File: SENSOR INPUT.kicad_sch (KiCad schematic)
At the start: 18 parts, among them J1 Screw_Terminal_01x02, J4 Screw_Terminal_01x03, U3 MAX31855KASA

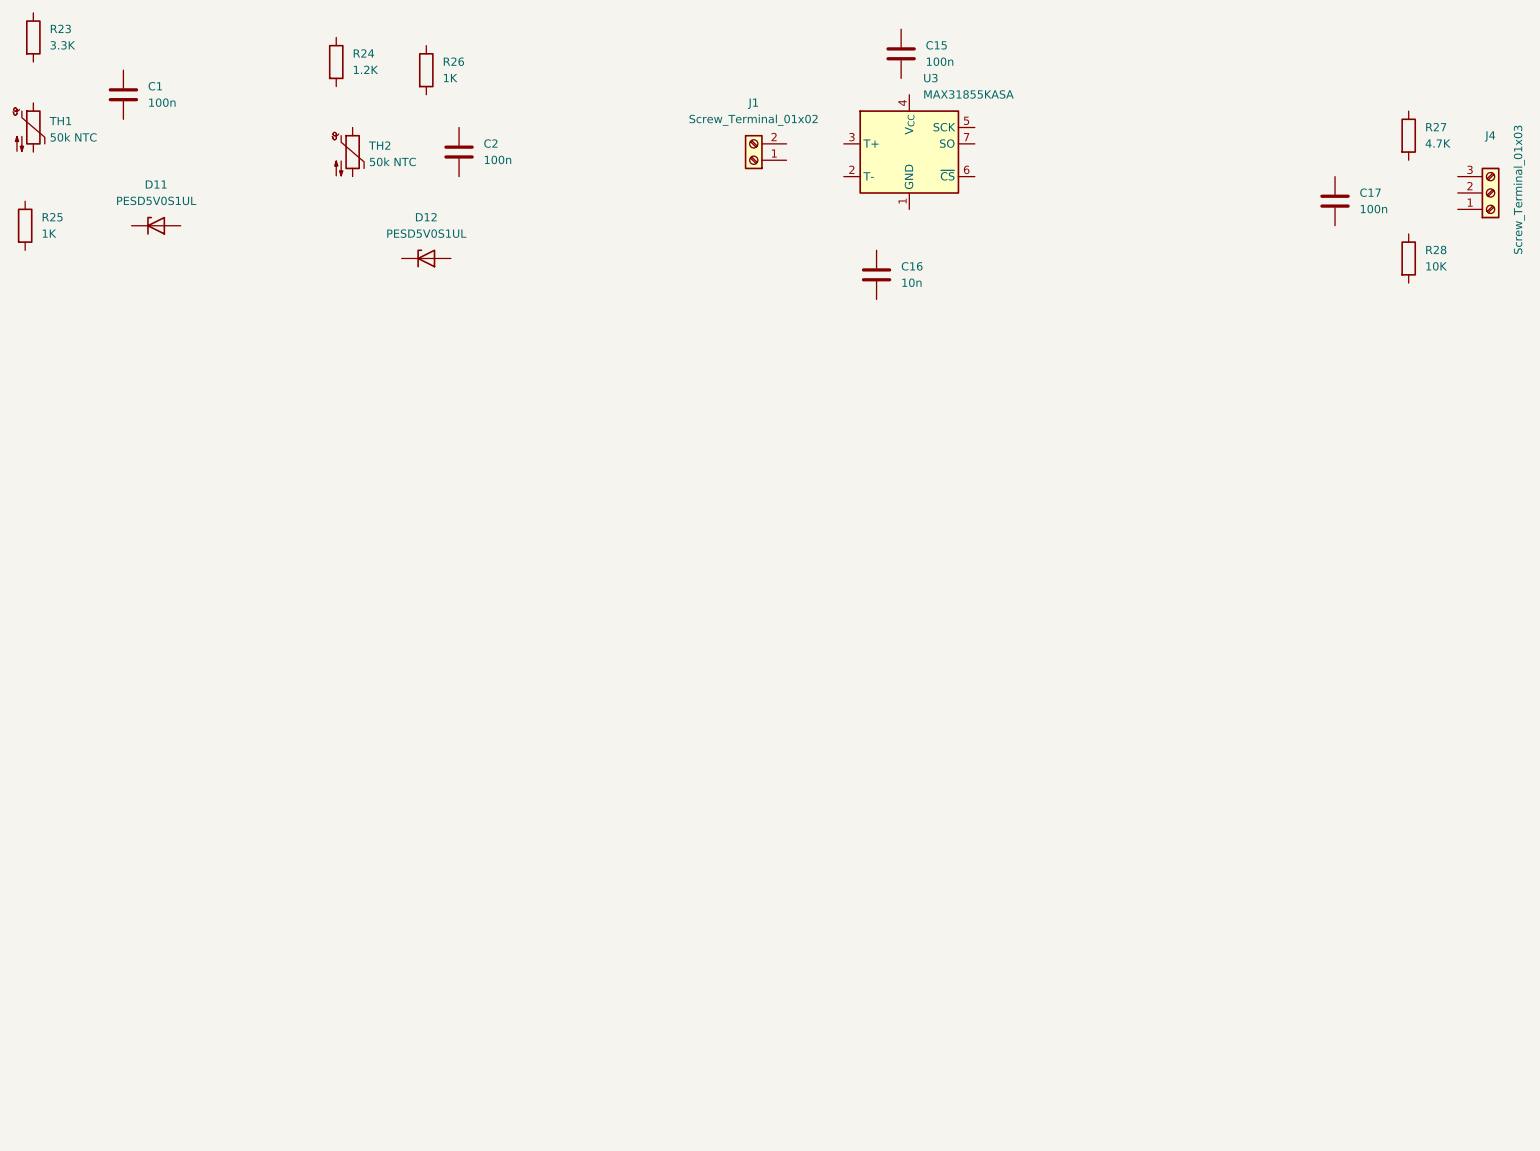
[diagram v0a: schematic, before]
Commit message: SCHEMATIC CONTINUATION
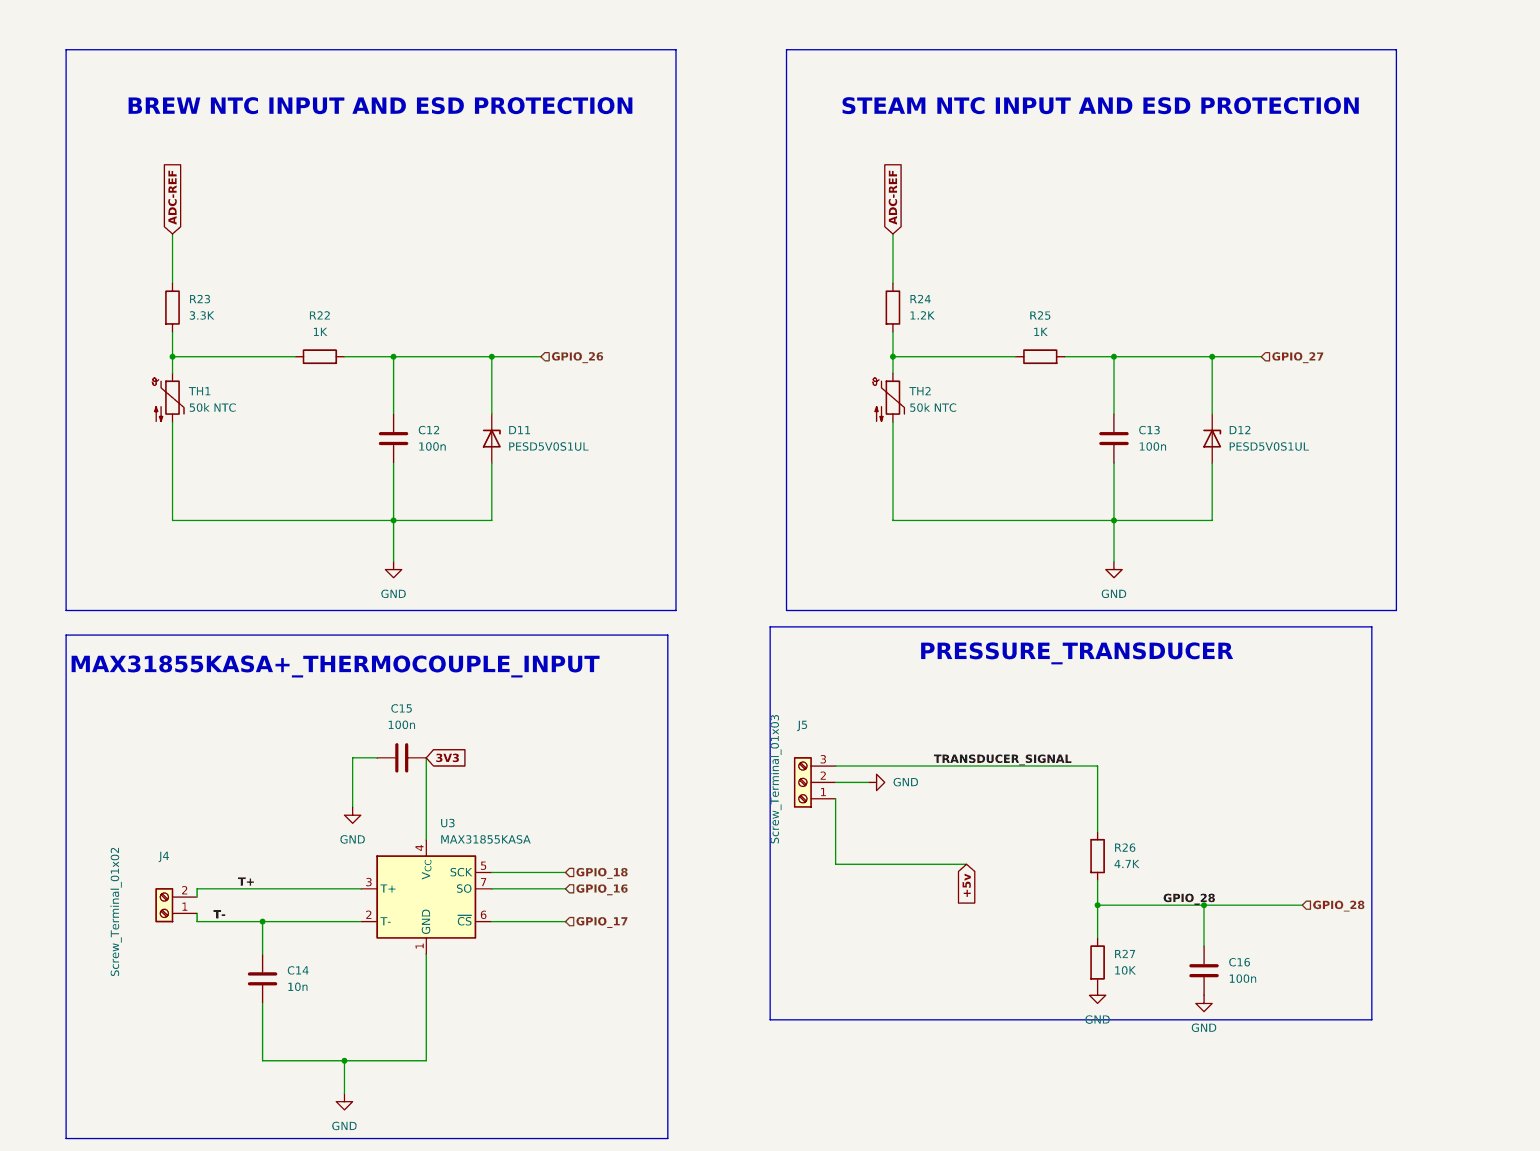
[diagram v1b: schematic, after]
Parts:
- removed C2: 100n, Capacitor_SMD:C_0805_2012Metric, symbol Device:C
- removed R26: 1K, Resistor_SMD:R_0805_2012Metric, symbol Device:R
- added C13: 100n, Capacitor_SMD:C_0805_2012Metric, symbol Device:C
- added R25: 1K, Resistor_SMD:R_0805_2012Metric, symbol Device:R
- renumbered C1 to C12, C16 to C14, C17 to C16, J1 to J4, J4 to J5, R25 to R22, R27 to R26, R28 to R27
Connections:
- net at R22.1: now also R23.2, TH1.1
- net GPIO_26: now reaches R22.2
- net GPIO_26: now also C12.1, D11.1 (K)
- net ADC-REF: now reaches R23.1
- net ADC-REF: now also R24.1
- net GPIO_28: now reaches C16.1
- net GPIO_28: now also R26.2, R27.1
- net GND: now reaches C16.2
- net GND: now also C12.2, C14.2, C15.1, D11.2 (A), D12.2 (A), J5.2 (Pin_2), R27.2, TH1.2, TH2.2, U3.1 (GND), C13.2
- net T-: now reaches J4.1 (Pin_1)
- net T-: now also C14.1, U3.2 (T-)
- net T+: now reaches J4.2 (Pin_2)
- net T+: now also U3.3 (T+)
- net TRANSDUCER_SIGNAL: now reaches R26.1
- net TRANSDUCER_SIGNAL: now also J5.3 (Pin_3)
- net 3V3: now reaches U3.4 (V_{CC})
- net 3V3: now also C15.2
- net GPIO_18: now reaches U3.5 (SCK)
- net GPIO_17: now reaches U3.6 (~{CS})
- net GPIO_16: now reaches U3.7 (SO)
- net GPIO_27: now reaches D12.1 (K)
- net GPIO_27: now also C13.1, R25.2
- net at R24.2: now also TH2.1, R25.1
- net +5v: now reaches J5.1 (Pin_1)
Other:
- note added: "BREW NTC INPUT AND ESD PROTECTION"
- note added: "MAX31855KASA+_THERMOCOUPLE_INPUT"
- note added: "PRESSURE_TRANSDUCER"
- note added: "STEAM NTC INPUT AND ESD PROTECTION"
- moved on the sheet: C12, C14, C15, C16, D11, J4, J5, R22, R23, R26, R27, TH1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
